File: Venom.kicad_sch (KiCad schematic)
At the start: 14 parts, among them CN1 HC-XH-5A-G, CN2 HC-PH-8A-G, CN3 HC-XH-8A-G, CN4 HC-XH-8A-G, CN5 HC-XH-2A-G, CN6 HC-PH-7A-G, SW1 GT-TC030A-H020-L1N, SW2 GT-TC030A-H020-L1N, U1 Pico

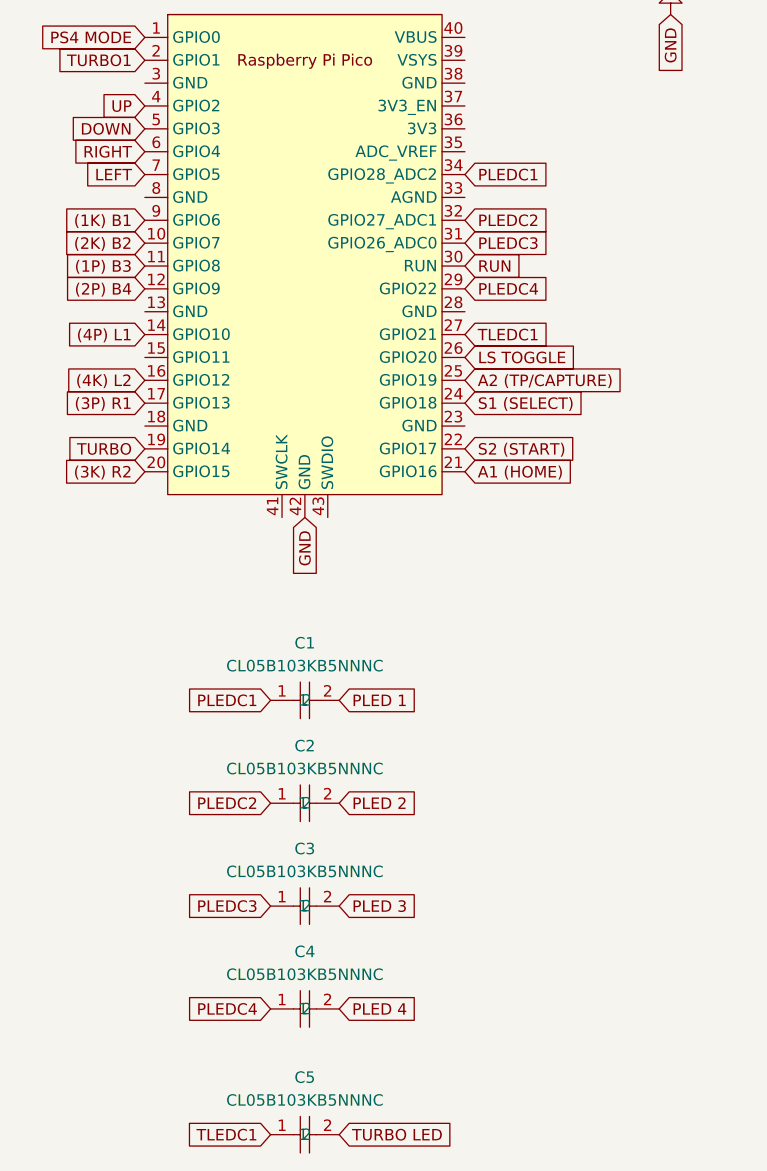
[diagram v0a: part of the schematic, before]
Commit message: LEDs need a resistor not capacitor?
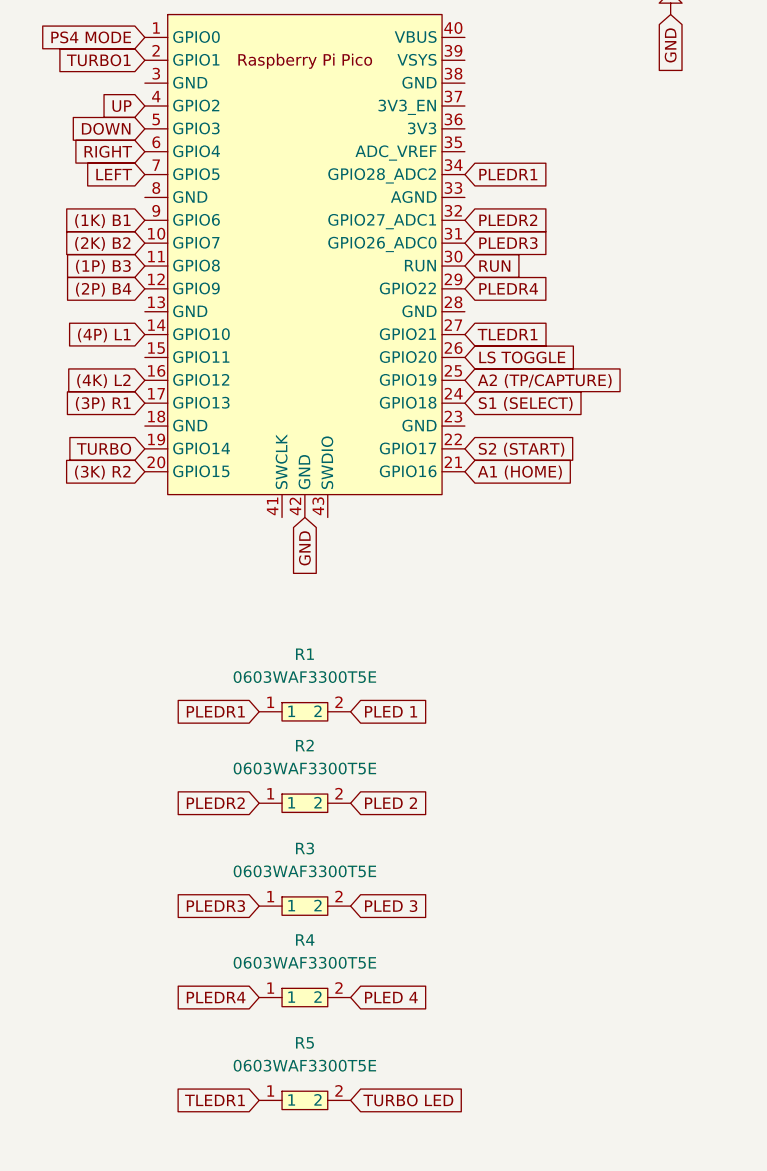
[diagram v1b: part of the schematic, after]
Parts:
- removed C1, C2, C3, C4, C5: CL05B103KB5NNNC, easyeda2kicad:C0402, symbol easyeda2kicad:CL05B103KB5NNNC
- added R1, R2, R3, R4, R5: 0603WAF3300T5E, easyeda2kicad:R0603, symbol easyeda2kicad:0603WAF3300T5E
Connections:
- net PLED 1: now also R1.2
- net PLED 2: now also R2.2
- net PLED 3: now also R3.2
- net PLED 4: now also R4.2
- net TURBO LED: now also R5.2
- net PLEDC1 renamed PLEDR1
- net PLEDR1: now also R1.1
- net PLEDC2 renamed PLEDR2
- net PLEDR2: now also R2.1
- net PLEDC3 renamed PLEDR3
- net PLEDR3: now also R3.1
- net PLEDC4 renamed PLEDR4
- net PLEDR4: now also R4.1
- net TLEDC1 renamed TLEDR1
- net TLEDR1: now also R5.1
